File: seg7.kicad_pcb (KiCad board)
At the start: 2 copper layers, 121.9 x 64.8 mm, 33 parts, among them U1 74HC595, U2 74HC595, U3 TD62083, U4 TD62083, U5 74HC595, U6 TD62083

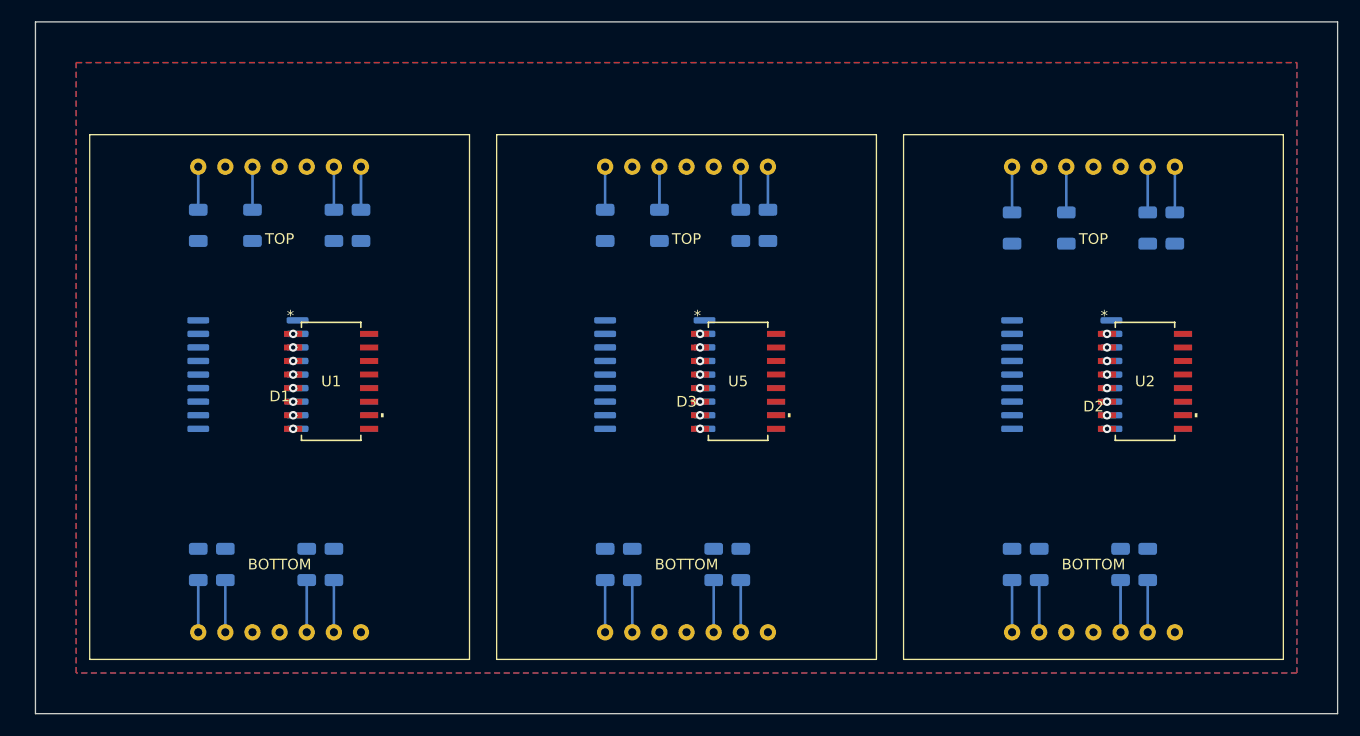
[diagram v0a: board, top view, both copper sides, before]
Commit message: update
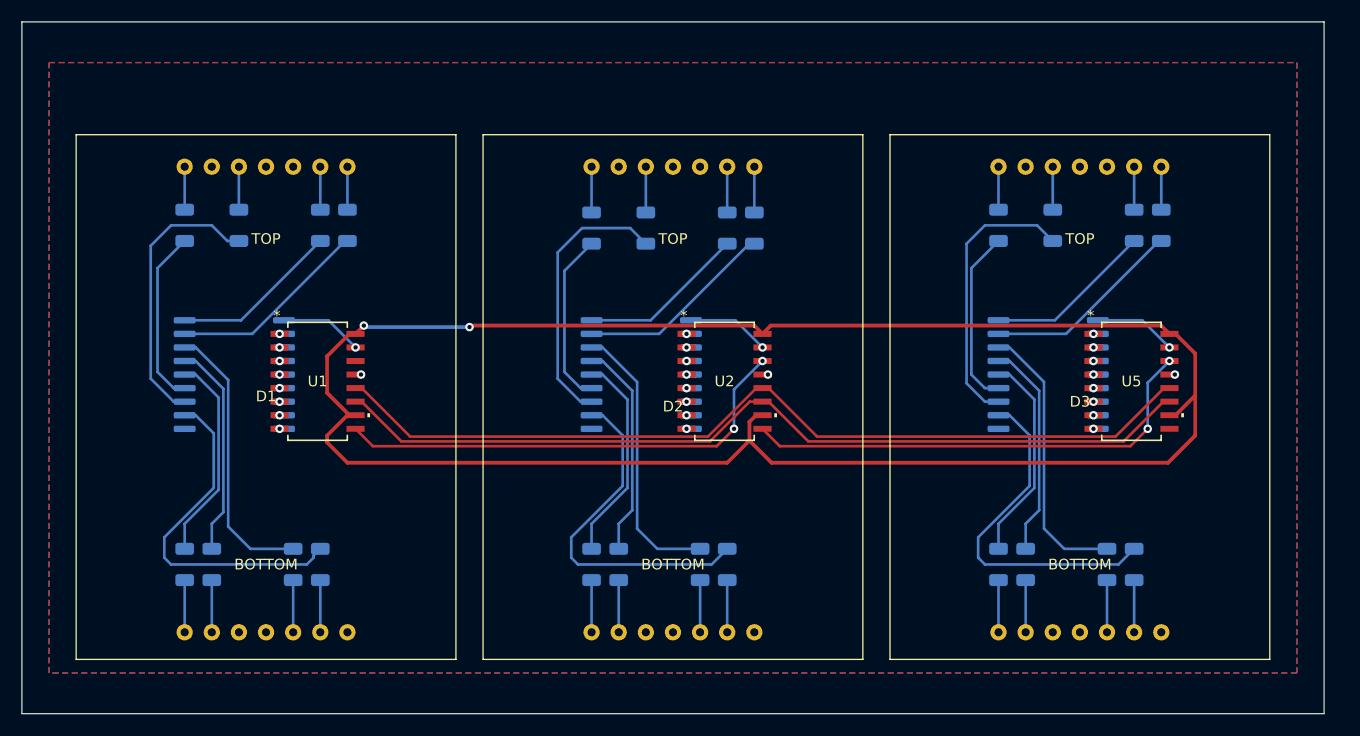
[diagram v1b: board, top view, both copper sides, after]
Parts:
- moved R10 39.4 mm to (124.5, 39.6)
- moved R11 39.4 mm to (124.5, 71.1)
- moved R12 39.4 mm to (127.0, 71.1)
- moved R13 39.4 mm to (137.2, 71.1)
- moved R14 39.4 mm to (134.6, 71.1)
- moved R15 39.4 mm to (139.7, 39.6)
- moved R16 39.4 mm to (137.2, 39.6)
- moved R9 39.4 mm to (129.5, 39.6)
- moved U2 39.4 mm to (136.9, 54.0)
- moved D2 39.4 mm to (132.1, 55.9)
- moved U4 39.4 mm to (129.1, 53.3)
- moved D3 36.8 mm to (170.2, 55.9)
- moved R22 36.8 mm to (172.7, 71.1)
- moved R23 36.8 mm to (177.8, 39.4)
- moved U5 36.8 mm to (175.0, 54.0)
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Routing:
- net +3.3V: track 0.00 -> 194.3 mm, vias 0 -> 2
- net RCLK: track 0.00 -> 83.7 mm
- net SRCLK: track 0.00 -> 82.4 mm
- net Net-(U2-QH'): track 0.00 -> 44.6 mm, vias 0 -> 2
- net Net-(U1-QH'): track 0.00 -> 44.2 mm, vias 0 -> 2
- net OUT24: track 0.00 -> 32.6 mm
- net OUT16: track 0.00 -> 32.6 mm
- net OUT8: track 0.00 -> 32.6 mm
- net OUT7: track 0.00 -> 26.2 mm
- net OUT23: track 0.00 -> 26.2 mm
- net OUT11: track 0.00 -> 26.0 mm
- net OUT19: track 0.00 -> 26.0 mm
- net OUT3: track 0.00 -> 26.0 mm
- net OUT15: track 0.00 -> 25.7 mm
- net OUT12: track 0.00 -> 20.3 mm
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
